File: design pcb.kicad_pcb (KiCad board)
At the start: 2 copper layers, 140 x 120 mm, 0 parts

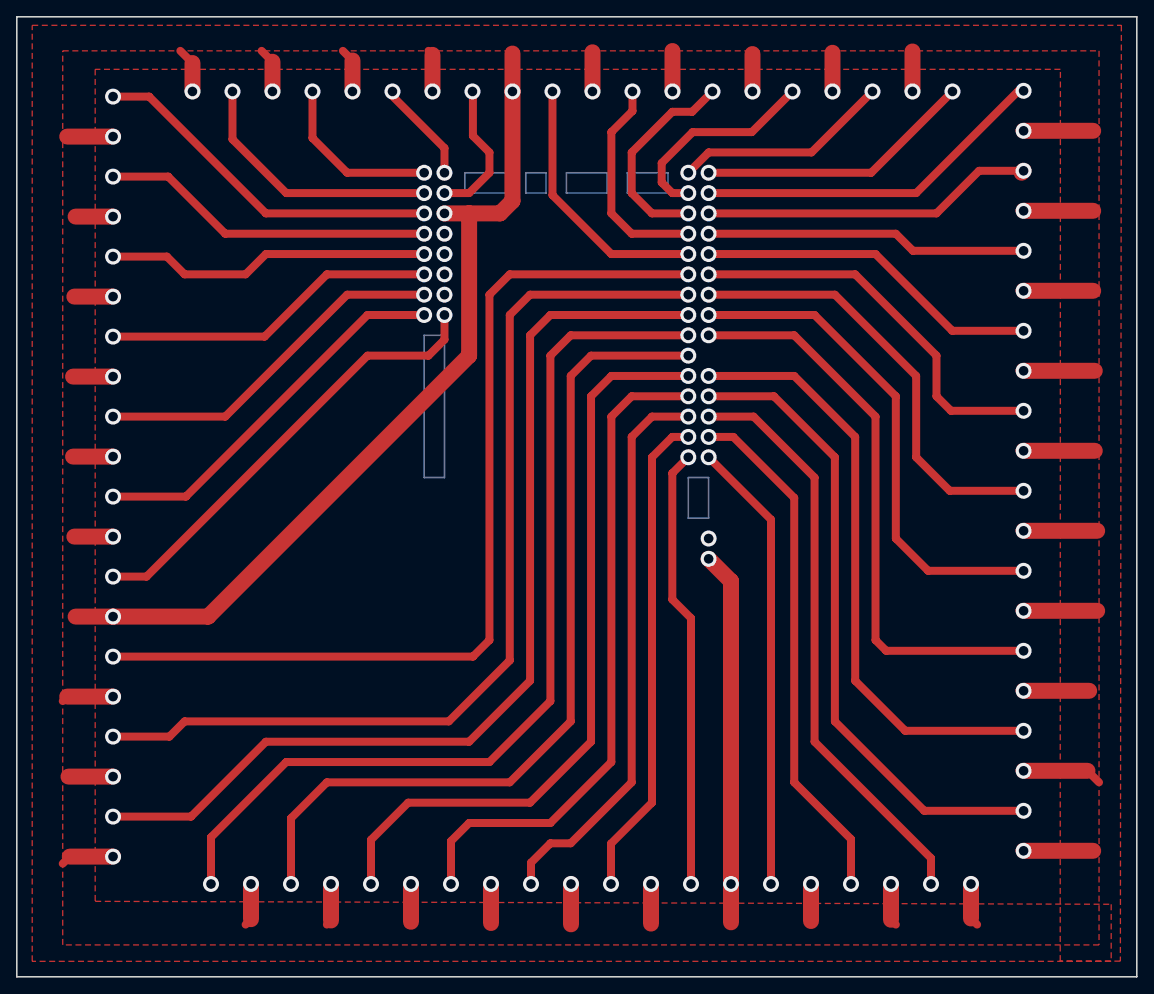
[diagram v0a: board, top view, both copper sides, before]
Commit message: v9
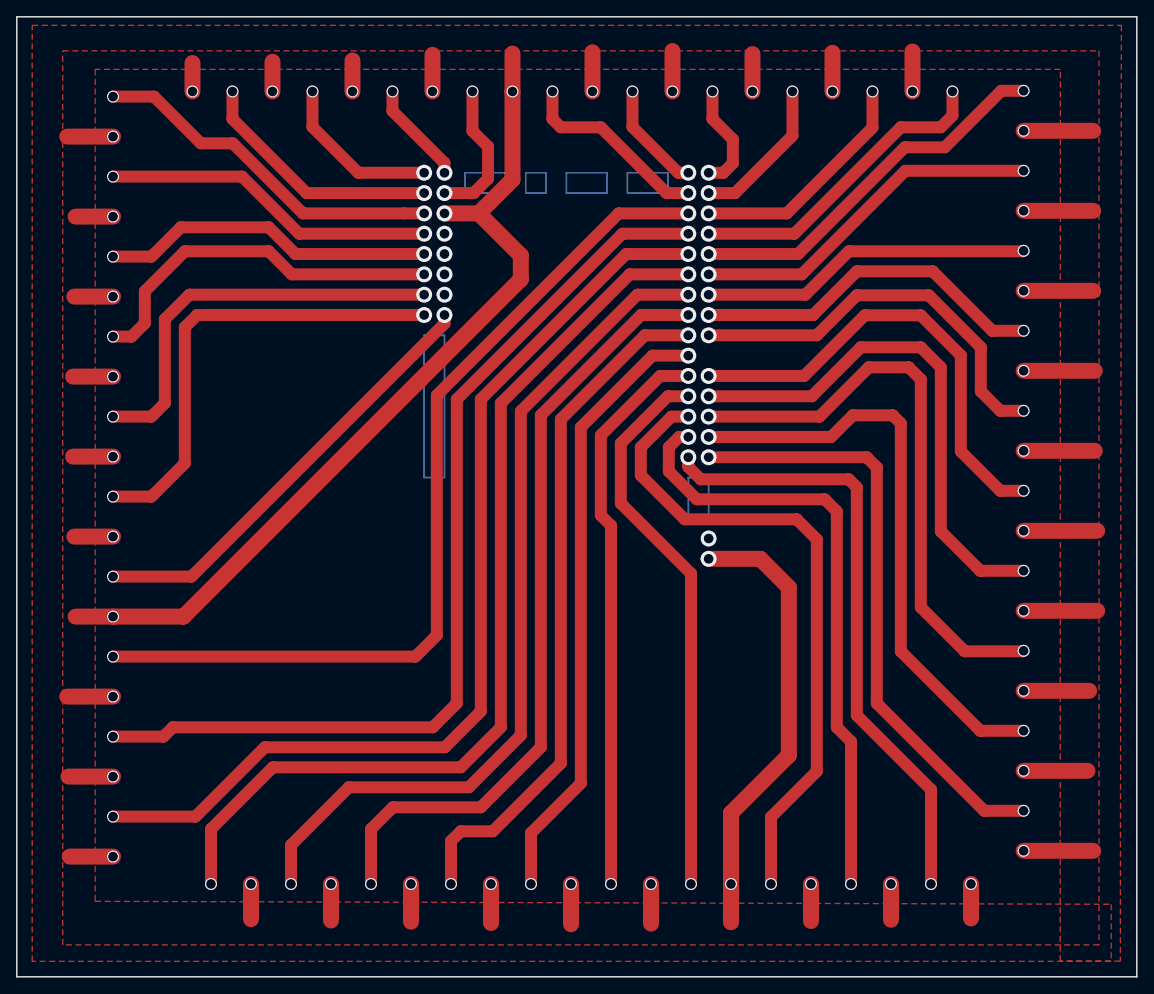
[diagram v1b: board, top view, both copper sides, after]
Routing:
- net (no net): track 2289.3 -> 2356.5 mm, vias 84 -> 85
- net GND: track 387.0 -> 382.1 mm, vias 43 -> 42
